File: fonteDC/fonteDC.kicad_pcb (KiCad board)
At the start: 2 copper layers, 184 x 150 mm, 18 parts, among them J1 Conn_01x02, T1 Transformer_1P_SS, U1 LM7805_TO220

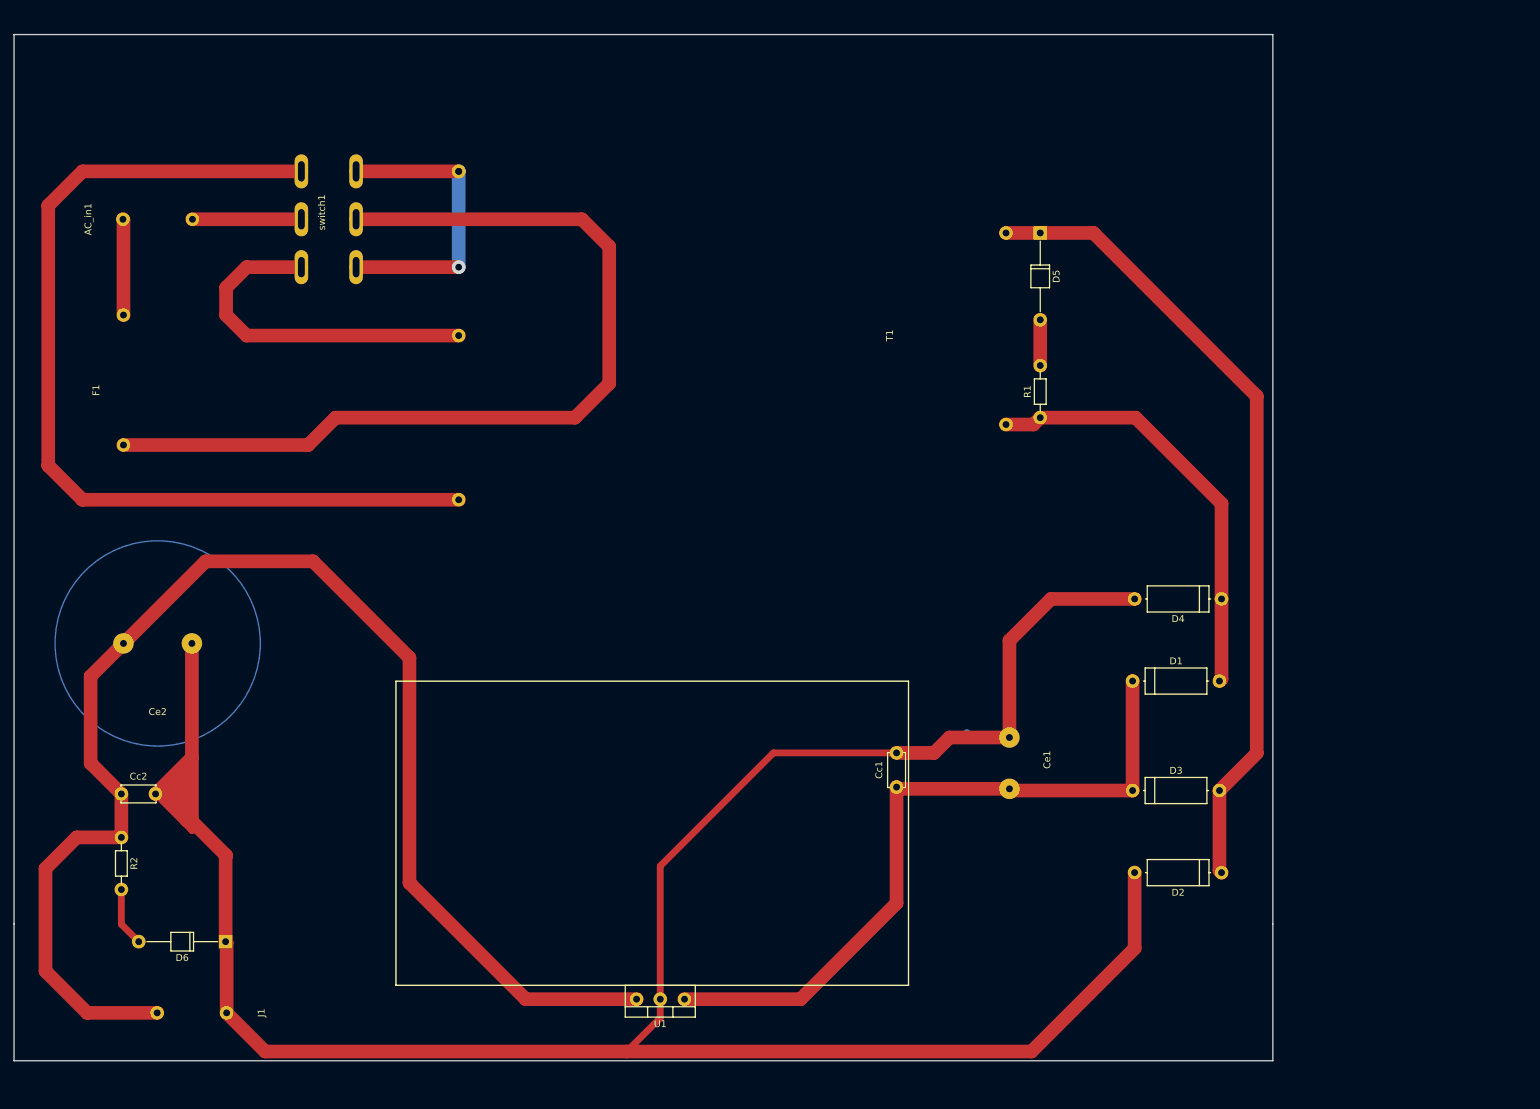
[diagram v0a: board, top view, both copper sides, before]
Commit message: First finished design.
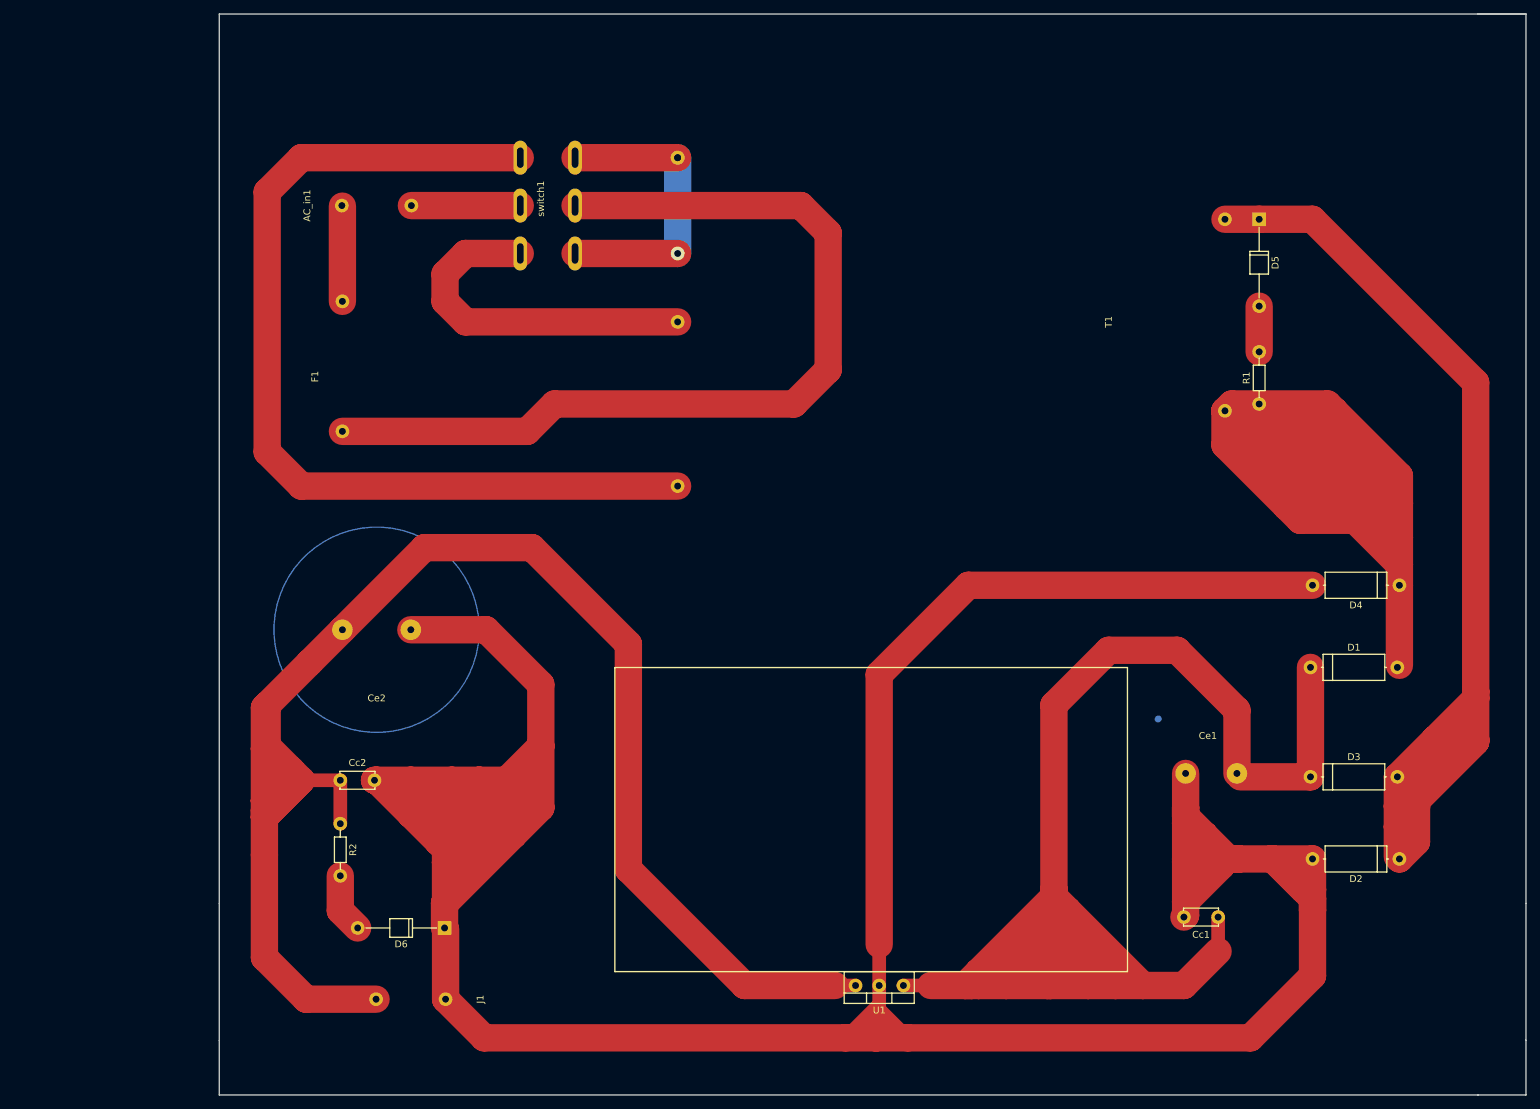
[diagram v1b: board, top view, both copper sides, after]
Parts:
- moved Cc1 50.7 mm to (192.0, 149.0), turned to 180 degrees
- moved Ce1 39.2 mm to (200.0, 128.0), turned to 180 degrees
- moved D6 32.1 mm to (78.9, 150.6)
- moved AC_in1 32.1 mm to (69.0, 45.0)
- moved Ce2 32.1 mm to (54.0, 107.0)
- moved D5 32.1 mm to (198.0, 47.0)
- moved F1 32.1 mm to (64.0, 56.0)
- moved J1 32.1 mm to (74.0, 161.0)
- moved R1 32.1 mm to (198.0, 74.0)
- moved T1 32.1 mm to (153.0, 106.0)
- moved U1 32.1 mm to (145.0, 159.0)
- moved switch1 32.1 mm to (94.0, 30.0)
- moved Cc2 32.1 mm to (63.7, 129.0)
- moved R2 32.1 mm to (63.7, 135.3)
- moved D1 26.1 mm to (205.5, 112.5)
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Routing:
- net Net-(D1-Pad2): track 63.2 -> 226.5 mm
- net Net-(Cc1-Pad2): track 416.6 -> 569.3 mm
- net Net-(Cc1-Pad1): track 105.5 -> 257.1 mm
- net Net-(D2-Pad1): track 120.8 -> 197.8 mm
- net Net-(Cc2-Pad1): track 205.5 -> 249.4 mm
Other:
- board size 184 x 150 mm -> 191 x 158 mm
- net class Default: trace_width 1 -> 4
- net class pwr added: clearance 1, trace_width 4, via_dia 2, via_drill 1
